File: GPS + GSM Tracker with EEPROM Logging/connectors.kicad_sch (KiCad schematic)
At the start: 15 parts, among them J2 Conn_01x04_Pin, J3 Conn_01x04_Pin, J4 Conn_01x02_Pin, J5 Conn_01x07_Pin, J6 Conn_01x04_Pin, J7 Conn_01x04_Pin, J8 Conn_01x07_Pin, SW1 SW_Push, SW2 SW_Push

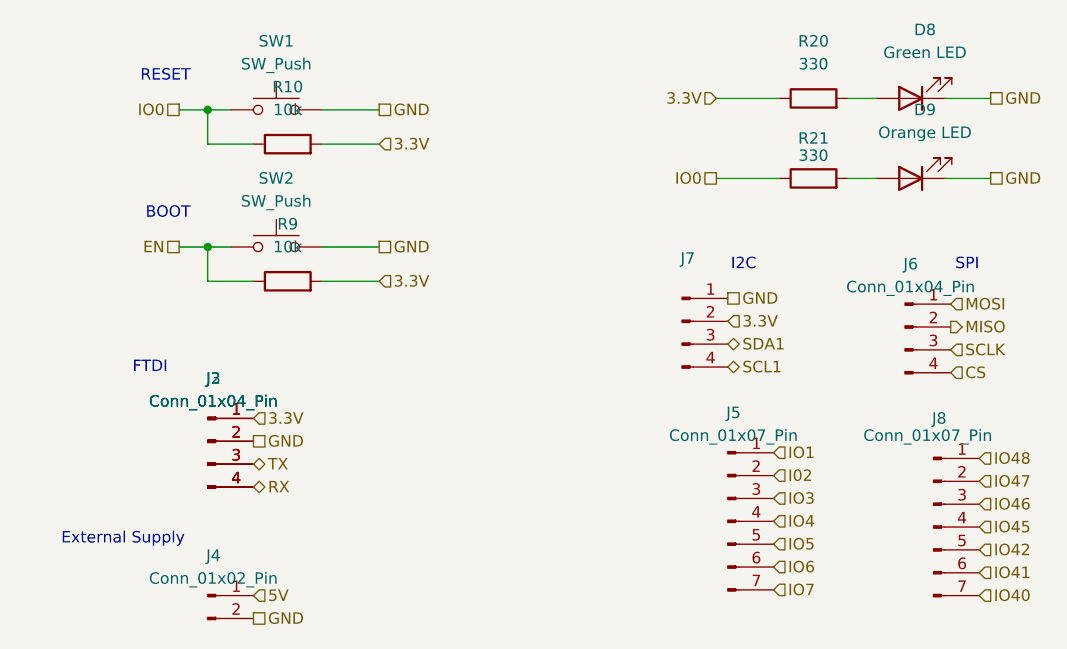
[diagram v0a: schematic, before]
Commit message: Completed Pcb design
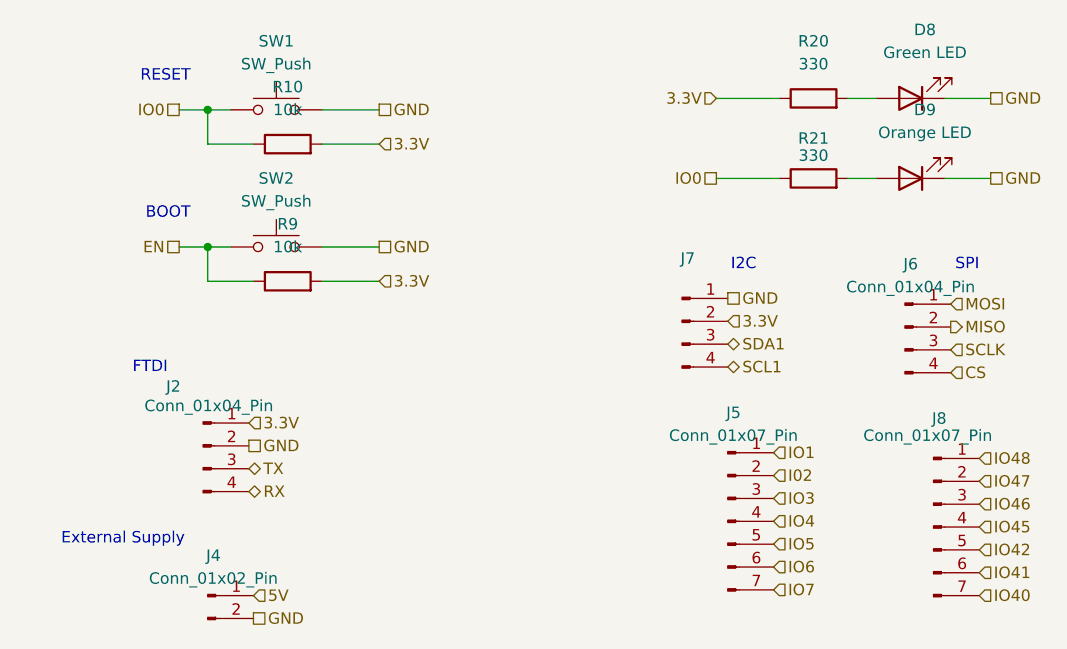
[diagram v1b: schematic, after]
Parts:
- removed J3: Conn_01x04_Pin, symbol Connector:Conn_01x04_Pin
- D8, D9: footprint (none) -> LED_SMD:LED_0805_2012Metric
- J2, J6, J7: footprint (none) -> Connector_Molex:Molex_KK-254_AE-6410-04A_1x04_P2.54mm_Vertical
- J4: footprint (none) -> Connector_Molex:Molex_KK-254_AE-6410-02A_1x02_P2.54mm_Vertical
- J5, J8: footprint (none) -> Connector_Molex:Molex_KK-254_AE-6410-07A_1x07_P2.54mm_Vertical
- R10, R20, R21, R9: footprint (none) -> Resistor_SMD:R_0805_2012Metric
- SW1, SW2: footprint (none) -> Button_Switch_THT:SW_PUSH_6mm_H4.3mm
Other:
- moved on the sheet: J2
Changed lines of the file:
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@@
 	(hierarchical_label "RX"
 		(shape bidirectional)
-		(at 49.53 73.66 0)
+		(at 49.022 74.168 0)
 		(effects
 			(font
@@
 	(hierarchical_label "TX"
 		(shape bidirectional)
-		(at 49.53 71.12 0)
+		(at 49.022 71.628 0)
 		(effects
 			(font
@@
 	(hierarchical_label "3.3V"
 		(shape input)
-		(at 49.53 66.04 0)
+		(at 49.022 66.548 0)
 		(effects
 			(font
@@
 	(hierarchical_label "GND"
 		(shape passive)
-		(at 49.53 68.58 0)
+		(at 49.022 69.088 0)
 		(effects
 			(font
@@
 			)
 		)
-		(property "Footprint" ""
+		(property "Footprint" "Resistor_SMD:R_0805_2012Metric"
 			(at 111.76 41.148 90)
 			(effects
@@
 			)
 		)
-		(property "Footprint" ""
+		(property "Footprint" "Resistor_SMD:R_0805_2012Metric"
 			(at 111.76 32.258 90)
 			(effects
@@
 			)
 		)
-		(property "Footprint" ""
+		(property "Footprint" "Connector_Molex:Molex_KK-254_AE-6410-04A_1x04_P2.54mm_Vertical"
 			(at 97.155 55.245 0)
 			(effects
@@
 			)
 		)
-		(property "Footprint" ""
+		(property "Footprint" "Button_Switch_THT:SW_PUSH_6mm_H4.3mm"
 			(at 52.07 41.91 0)
 			(effects
@@
 			)
 		)
-		(property "Footprint" ""
+		(property "Footprint" "Connector_Molex:Molex_KK-254_AE-6410-02A_1x02_P2.54mm_Vertical"
 			(at 44.45 85.725 0)
 			(effects
@@
 				(path "/98ceb1ac-bd30-43a6-9b0c-d172f1189100/f04a2659-cc82-4231-96d1-5a6a6e2ef39d"
 					(reference "J4")
-					(unit 1)
-				)
-			)
-		)
-	)
-	(symbol
-		(lib_id "Connector:Conn_01x04_Pin")
-		(at 44.45 68.58 0)
-		(unit 1)
-		(exclude_from_sim no)
-		(in_bom yes)
-		(on_board yes)
-		(dnp no)
-		(fields_autoplaced yes)
-		(property "Reference" "J3"
-			(at 45.085 61.595 0)
-			(effects
-				(font
-					(size 1.27 1.27)
-				)
-			)
-		)
-		(property "Value" "Conn_01x04_Pin"
-			(at 45.085 64.135 0)
-			(effects
-				(font
-					(size 1.27 1.27)
-				)
-			)
-		)
-		(property "Footprint" ""
-			(at 44.45 68.58 0)
-			(effects
-				(font
-					(size 1.27 1.27)
-				)
-				(hide yes)
-			)
-		)
-		(property "Datasheet" "~"
-			(at 44.45 68.58 0)
-			(effects
-				(font
-					(size 1.27 1.27)
-				)
-				(hide yes)
-			)
-		)
-		(property "Description" "Generic connector, single row, 01x04, script generated"
-			(at 44.45 68.58 0)
-			(effects
-				(font
-					(size 1.27 1.27)
-				)
-				(hide yes)
-			)
-		)
-		(pin "1"
-		)
-		(pin "2"
-		)
-		(pin "4"
-		)
-		(pin "3"
-		)
-		(instances
-			(project ""
-				(path "/98ceb1ac-bd30-43a6-9b0c-d172f1189100/f04a2659-cc82-4231-96d1-5a6a6e2ef39d"
-					(reference "J3")
 					(unit 1)
 				)
@@
 			)
 		)
-		(property "Footprint" ""
+		(property "Footprint" "LED_SMD:LED_0805_2012Metric"
 			(at 122.555 39.37 0)
 			(effects
@@
 			)
 		)
-		(property "Footprint" ""
+		(property "Footprint" "Button_Switch_THT:SW_PUSH_6mm_H4.3mm"
 			(at 52.07 26.67 0)
 			(effects
@@
 			)
 		)
-		(property "Footprint" ""
+		(property "Footprint" "Connector_Molex:Molex_KK-254_AE-6410-04A_1x04_P2.54mm_Vertical"
 			(at 121.92 55.88 0)
 			(effects
@@
 			)
 		)
-		(property "Footprint" ""
+		(property "Footprint" "Connector_Molex:Molex_KK-254_AE-6410-07A_1x07_P2.54mm_Vertical"
 			(at 102.235 77.47 0)
 			(effects
@@
 			)
 		)
-		(property "Footprint" ""
+		(property "Footprint" "Resistor_SMD:R_0805_2012Metric"
 			(at 53.34 37.338 90)
 			(effects
@@
 			)
 		)
-		(property "Footprint" ""
+		(property "Footprint" "Connector_Molex:Molex_KK-254_AE-6410-07A_1x07_P2.54mm_Vertical"
 			(at 125.095 78.105 0)
 			(effects
@@
 	(symbol
 		(lib_id "Connector:Conn_01x04_Pin")
-		(at 44.45 68.58 0)
-		(unit 1)
-		(exclude_from_sim no)
-		(in_bom yes)
-		(on_board yes)
-		(dnp no)
-		(fields_autoplaced yes)
+		(at 43.942 69.088 0)
+		(unit 1)
+		(exclude_from_sim no)
+		(in_bom yes)
+		(on_board yes)
+		(dnp no)
 		(property "Reference" "J2"
-			(at 45.085 61.595 0)
+			(at 40.64 62.484 0)
 			(effects
 				(font
@@
 		)
 		(property "Value" "Conn_01x04_Pin"
-			(at 45.085 64.135 0)
-			(effects
-				(font
-					(size 1.27 1.27)
-				)
-			)
-		)
-		(property "Footprint" ""
-			(at 44.45 68.58 0)
-			(effects
-				(font
-					(size 1.27 1.27)
-				)
-				(hide yes)
-			)
-		)
-		(property "Datasheet" "~"
-			(at 44.45 68.58 0)
+			(at 44.577 64.643 0)
+			(effects
+				(font
+					(size 1.27 1.27)
+				)
+			)
+		)
+		(property "Footprint" "Connector_Molex:Molex_KK-254_AE-6410-04A_1x04_P2.54mm_Vertical"
+			(at 43.942 69.088 0)
+			(effects
+				(font
+					(size 1.27 1.27)
+				)
+				(hide yes)
+			)
+		)
+		(property "Datasheet" "~"
+			(at 43.942 69.088 0)
 			(effects
 				(font
@@
 		)
 		(property "Description" "Generic connector, single row, 01x04, script generated"
-			(at 44.45 68.58 0)
+			(at 43.942 69.088 0)
 			(effects
 				(font
@@
 			)
 		)
-		(property "Footprint" ""
+		(property "Footprint" "LED_SMD:LED_0805_2012Metric"
 			(at 122.555 30.48 0)
 			(effects
@@
 			)
 		)
-		(property "Footprint" ""
+		(property "Footprint" "Resistor_SMD:R_0805_2012Metric"
 			(at 53.34 52.578 90)
 			(effects
